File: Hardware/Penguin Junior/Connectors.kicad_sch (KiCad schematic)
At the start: 34 parts, among them J1 USB_B_Micro, J10 Conn_01x06_UART, J10 Conn_01x10, J11 Conn_01x06_UART, J11 Conn_01x10, J12 Conn_01x10, J14 Conn_01x04_UART, J16 Conn_02x05_SWD, J2 Conn_01x03_Video, J2 Micro_SD_Card_Det1, J5 Conn_01x03_Video, J9 Conn_01x04_I2C

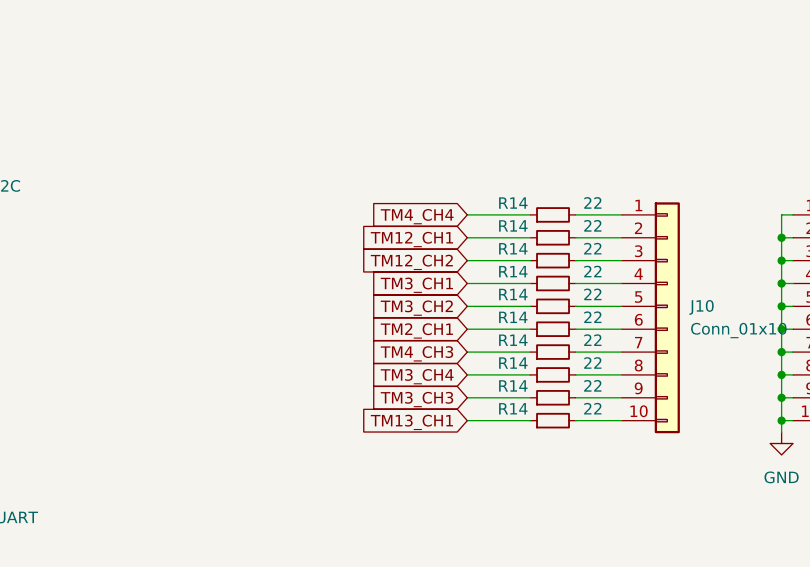
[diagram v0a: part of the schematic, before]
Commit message: Updated Penguin project
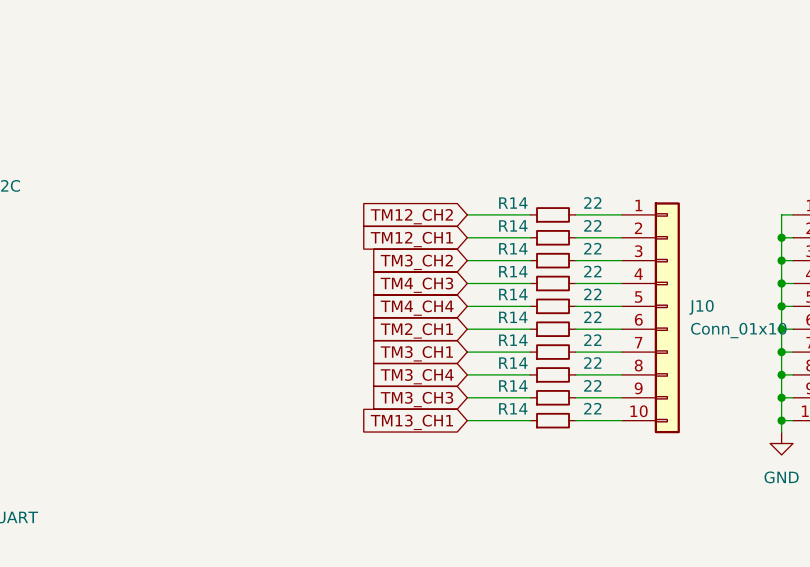
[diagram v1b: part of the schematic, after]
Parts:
- R2: footprint Resistor_SMD:R_0603_1608Metric -> Resistor_SMD:R_0402_1005Metric
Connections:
- net TM12_CH2: now also R14.1; no longer R14.1
- net TM3_CH1: now also R14.1; no longer R14.1
- net TM3_CH2: now also R14.1; no longer R14.1
- net TM4_CH3: now also R14.1; no longer R14.1
- net TM4_CH4: now also R14.1; no longer R14.1

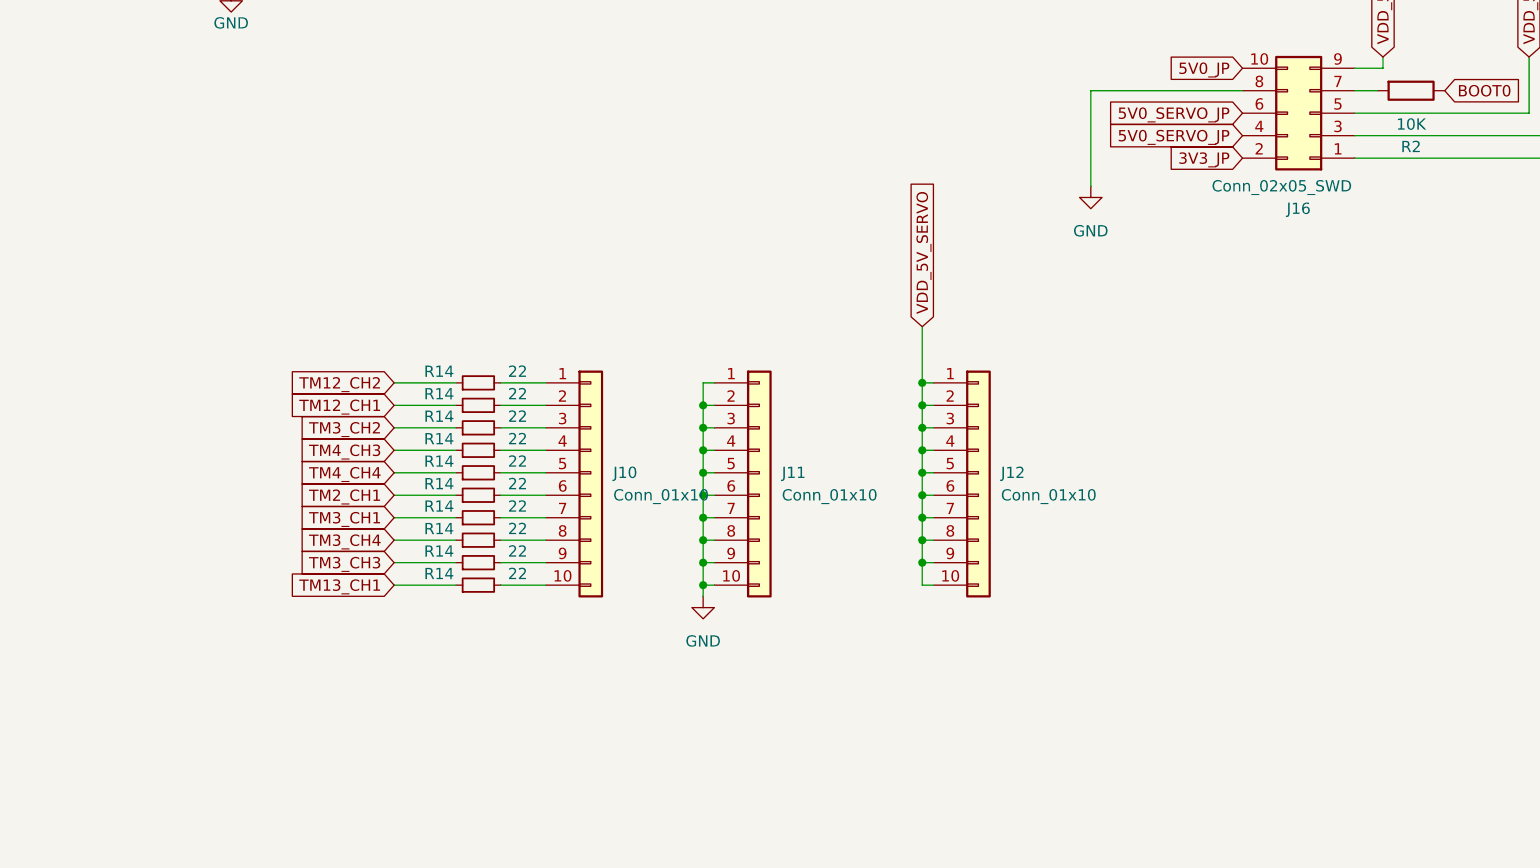
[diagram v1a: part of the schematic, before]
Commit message: Updated Penguin project
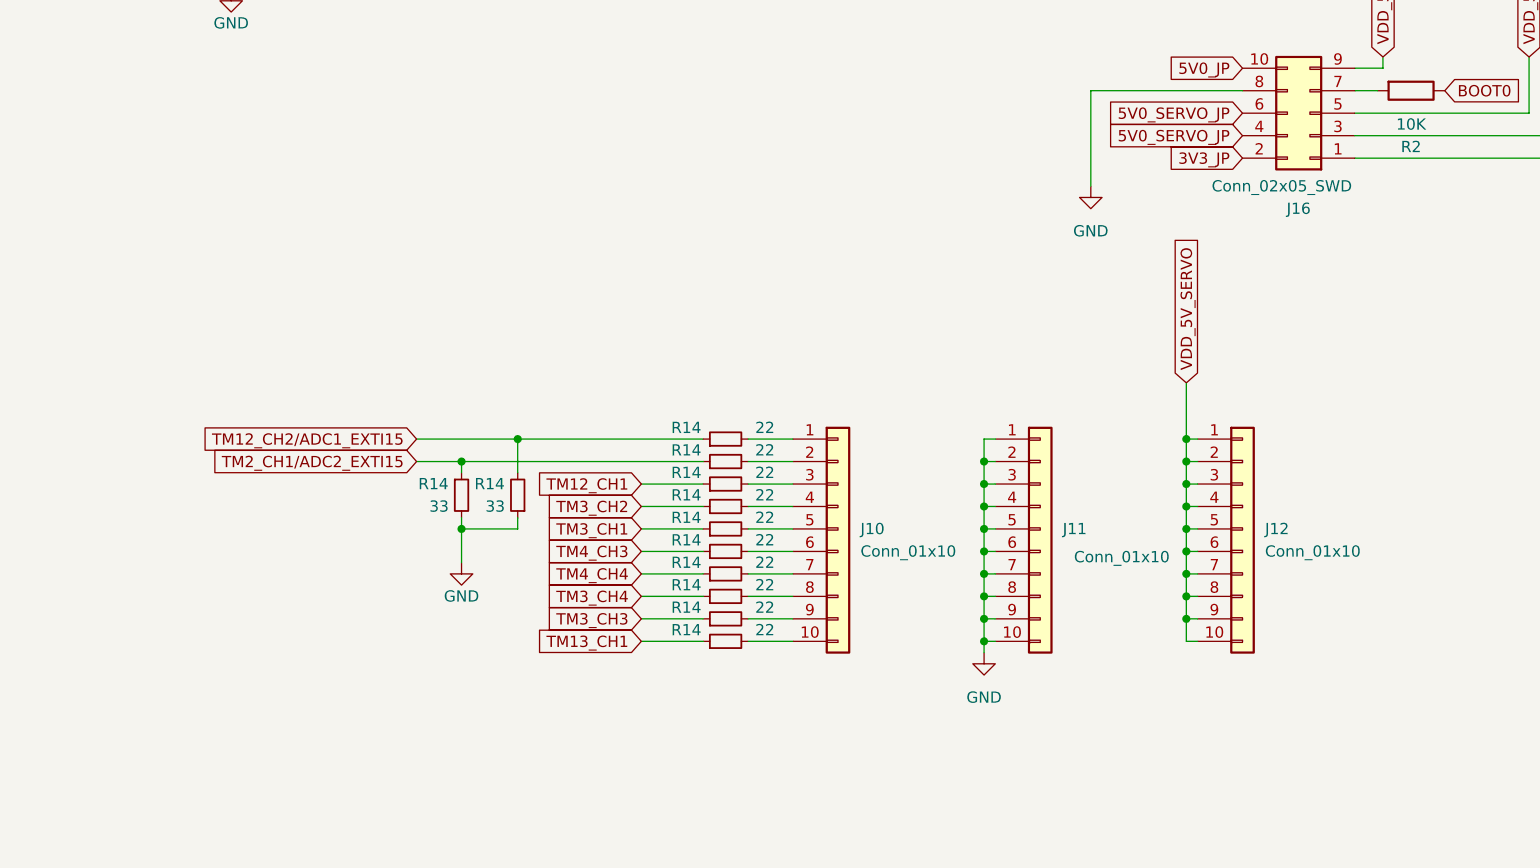
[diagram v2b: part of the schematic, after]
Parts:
- added R14 (x2): 33, Resistor_SMD:R_0402_1005Metric, symbol Device:R_Small
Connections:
- net GND: now also R14.1, R14.2
- net at R14.2: now also J10.2 (Pin_2); no longer J10.6 (Pin_6)
- net at R14.2: now also J10.4 (Pin_4); no longer J10.3 (Pin_3)
- net at R14.2: now also J10.3 (Pin_3); no longer J10.2 (Pin_2)
- net at R14.2: now also J10.6 (Pin_6); no longer J10.4 (Pin_4)
- net at J10.5 (Pin_5): now also R14.2; no longer R14.2
- net at J10.7 (Pin_7): now also R14.2; no longer R14.2
- net TM12_CH2 renamed TM12_CH2/ADC1_EXTI15
- net TM12_CH2/ADC1_EXTI15: now also R14.2
- net TM2_CH1 renamed TM2_CH1/ADC2_EXTI15
- net TM2_CH1/ADC2_EXTI15: now also R14.1
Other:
- moved on the sheet: J10, J11, J12, R14

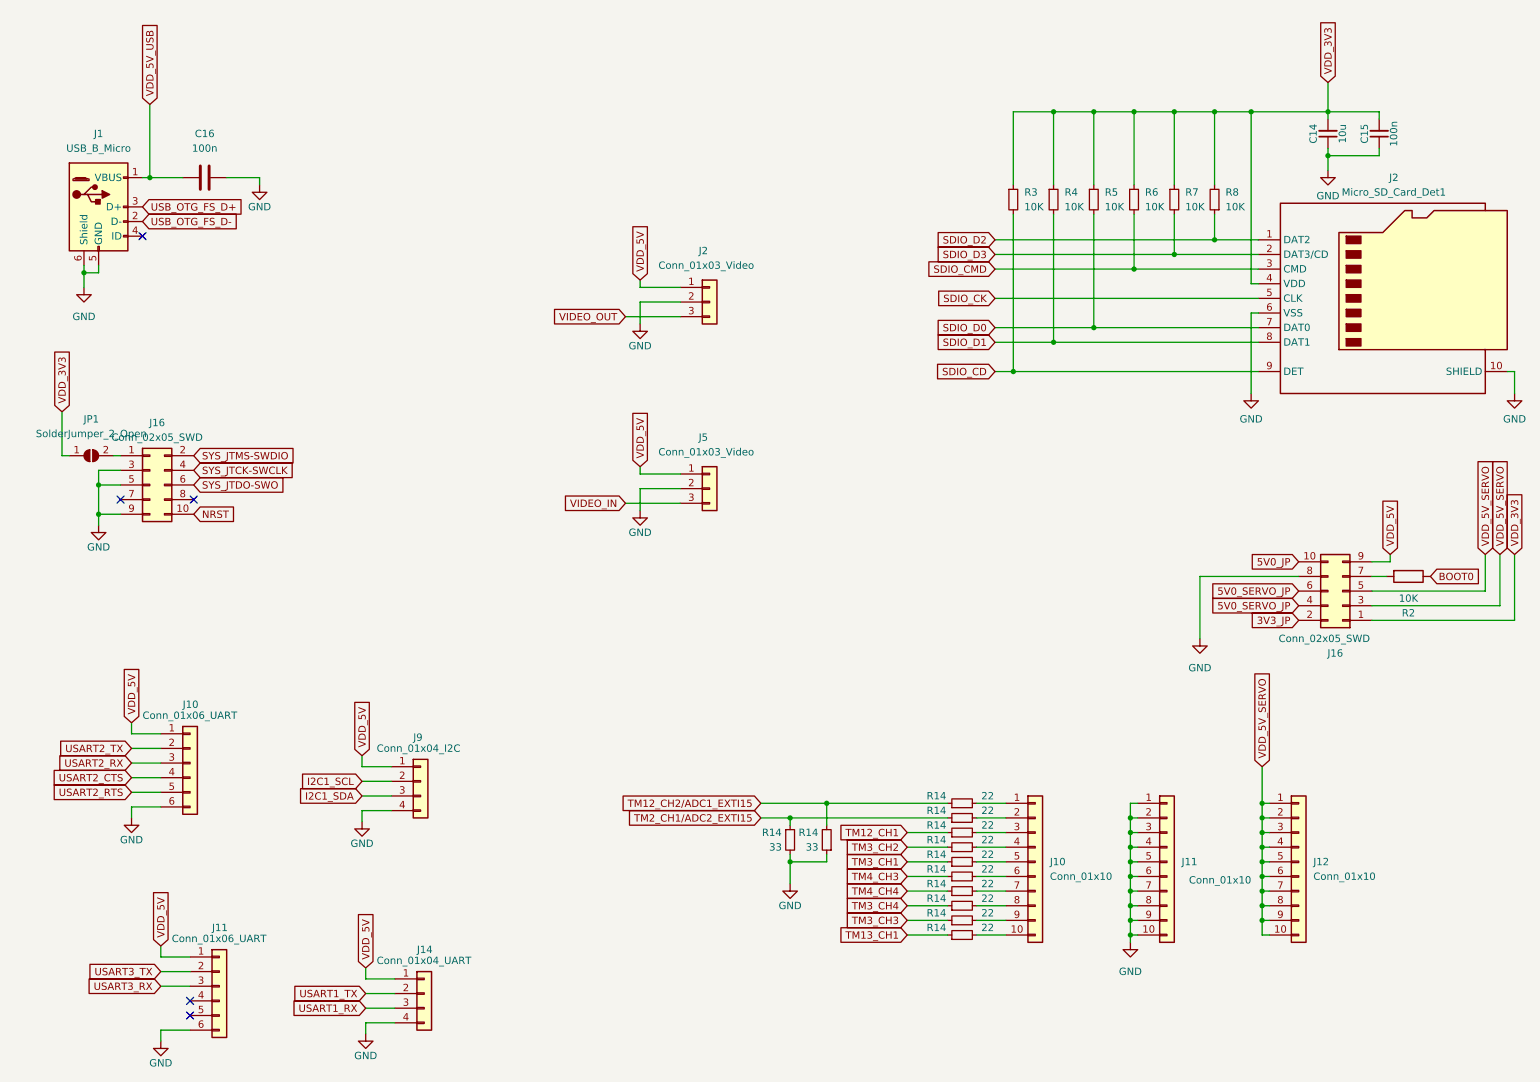
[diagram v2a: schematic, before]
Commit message: Updated Penguin project
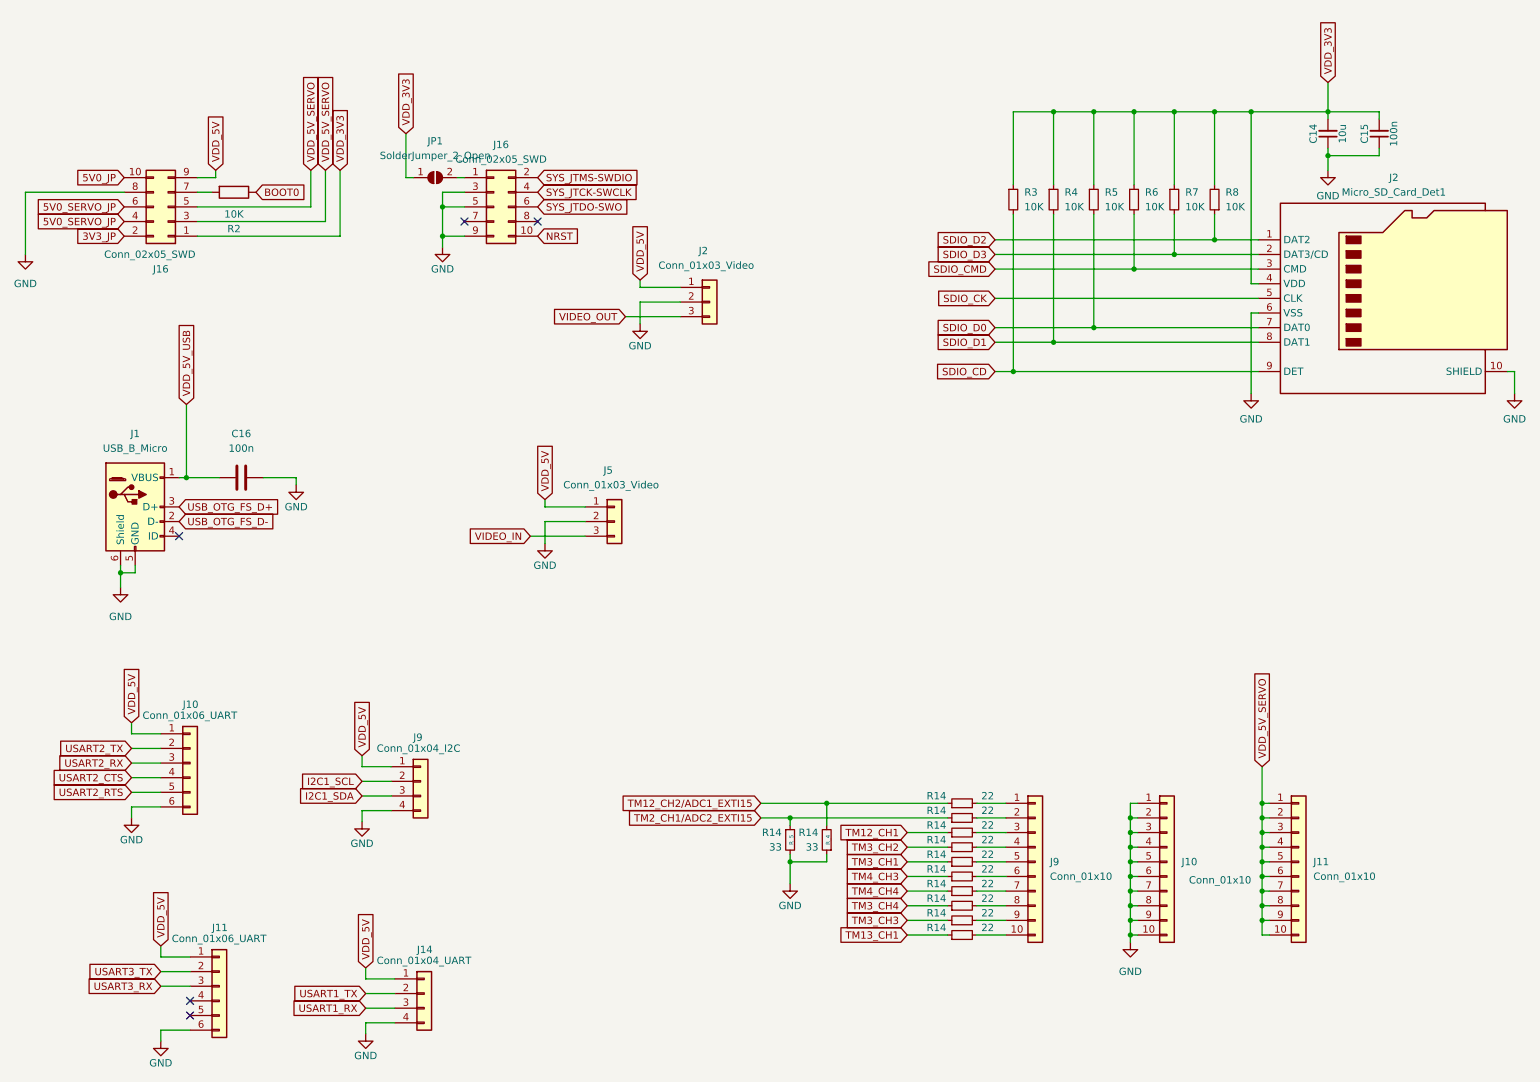
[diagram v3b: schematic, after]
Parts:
- JP1: footprint Jumper:SolderJumper-2_P1.3mm_Open_Pad1.0x1.5mm -> Jumper:SolderJumper-2_P1.3mm_Open_RoundedPad1.0x1.5mm
- renumbered J11 to J10, J12 to J11, J10 to J9
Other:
- note added: "R_4"
- note added: "R_5"
- moved on the sheet: C16, J1, J16, J5, JP1, R2
